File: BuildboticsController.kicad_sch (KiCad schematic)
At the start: 0 parts

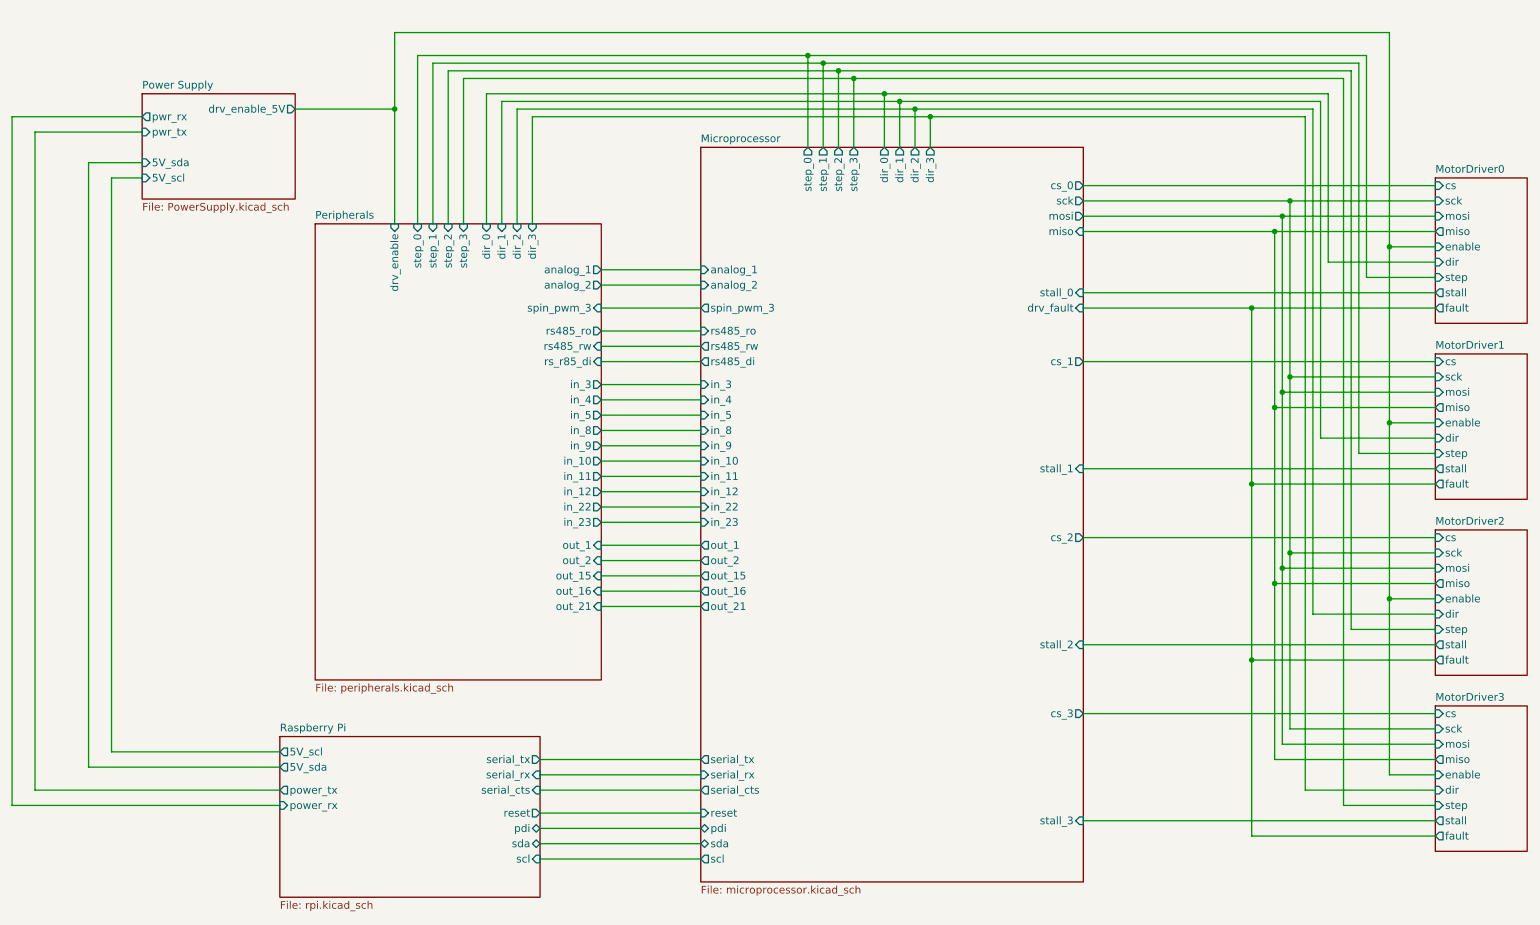
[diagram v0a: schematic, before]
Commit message: first commit of V18
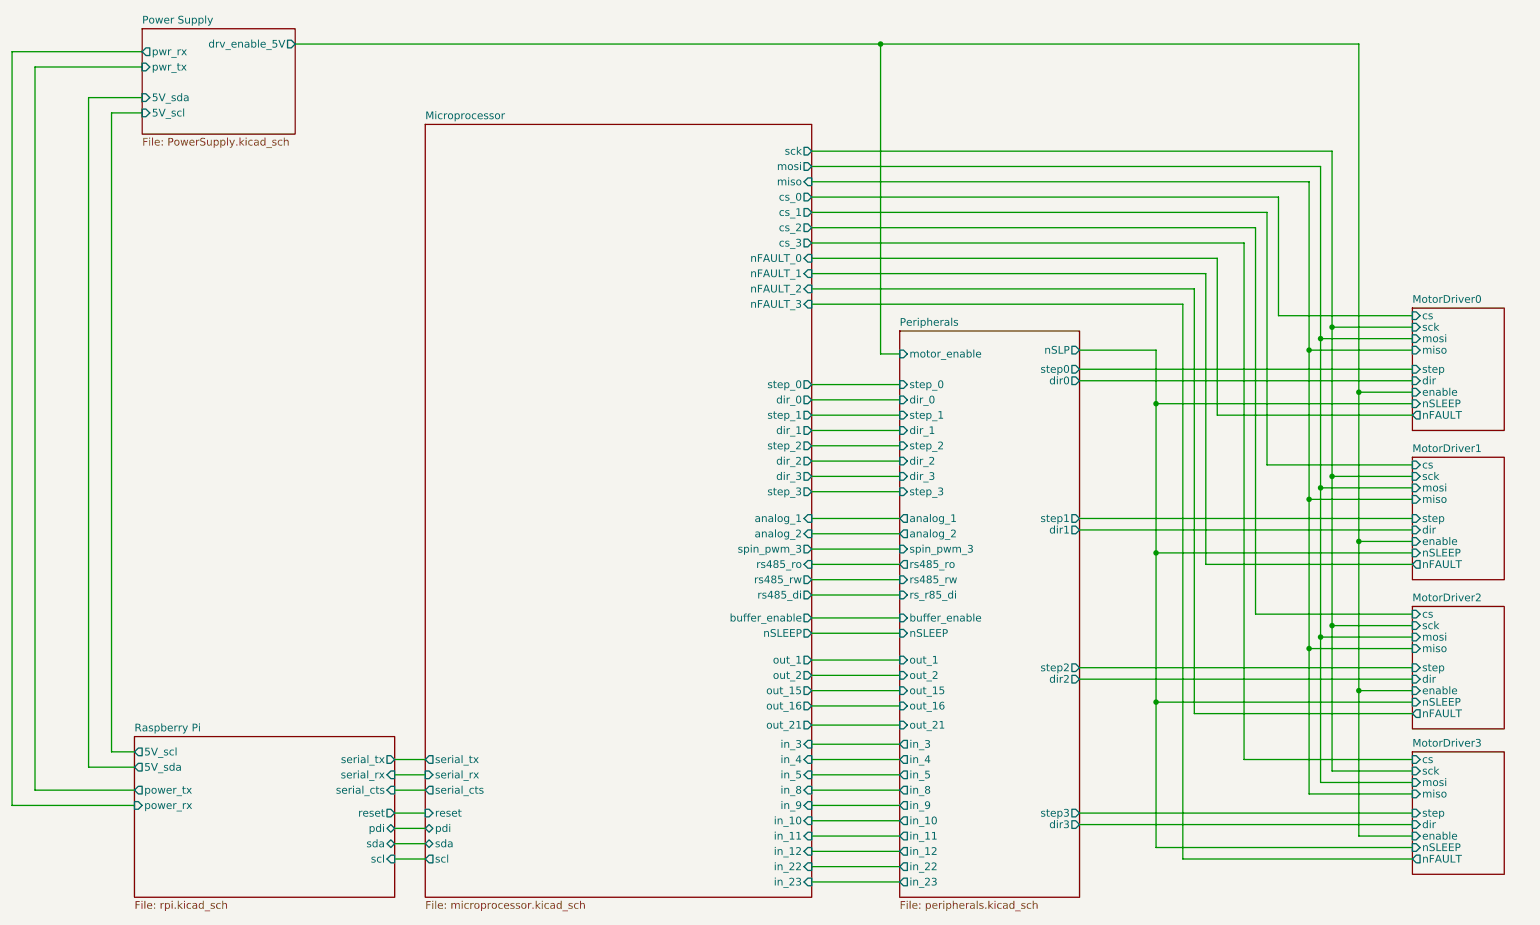
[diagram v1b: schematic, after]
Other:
- sheet Microprocessor ports: added buffer_enable, nFAULT_0, nFAULT_1, nFAULT_2, nFAULT_3, nSLEEP; removed drv_fault, stall_0, stall_1, stall_2, stall_3
- sheet MotorDriver0 ports: added nFAULT, nSLEEP; removed fault, stall
- sheet MotorDriver1 ports: added nFAULT, nSLEEP; removed fault, stall
- sheet MotorDriver2 ports: added nFAULT, nSLEEP; removed fault, stall
- sheet MotorDriver3 ports: added nFAULT, nSLEEP; removed fault, stall
- sheet Peripherals ports: added buffer_enable, dir0, dir1, dir2, dir3, motor_enable, nSLEEP, nSLP, step0, step1, step2, step3; removed drv_enable

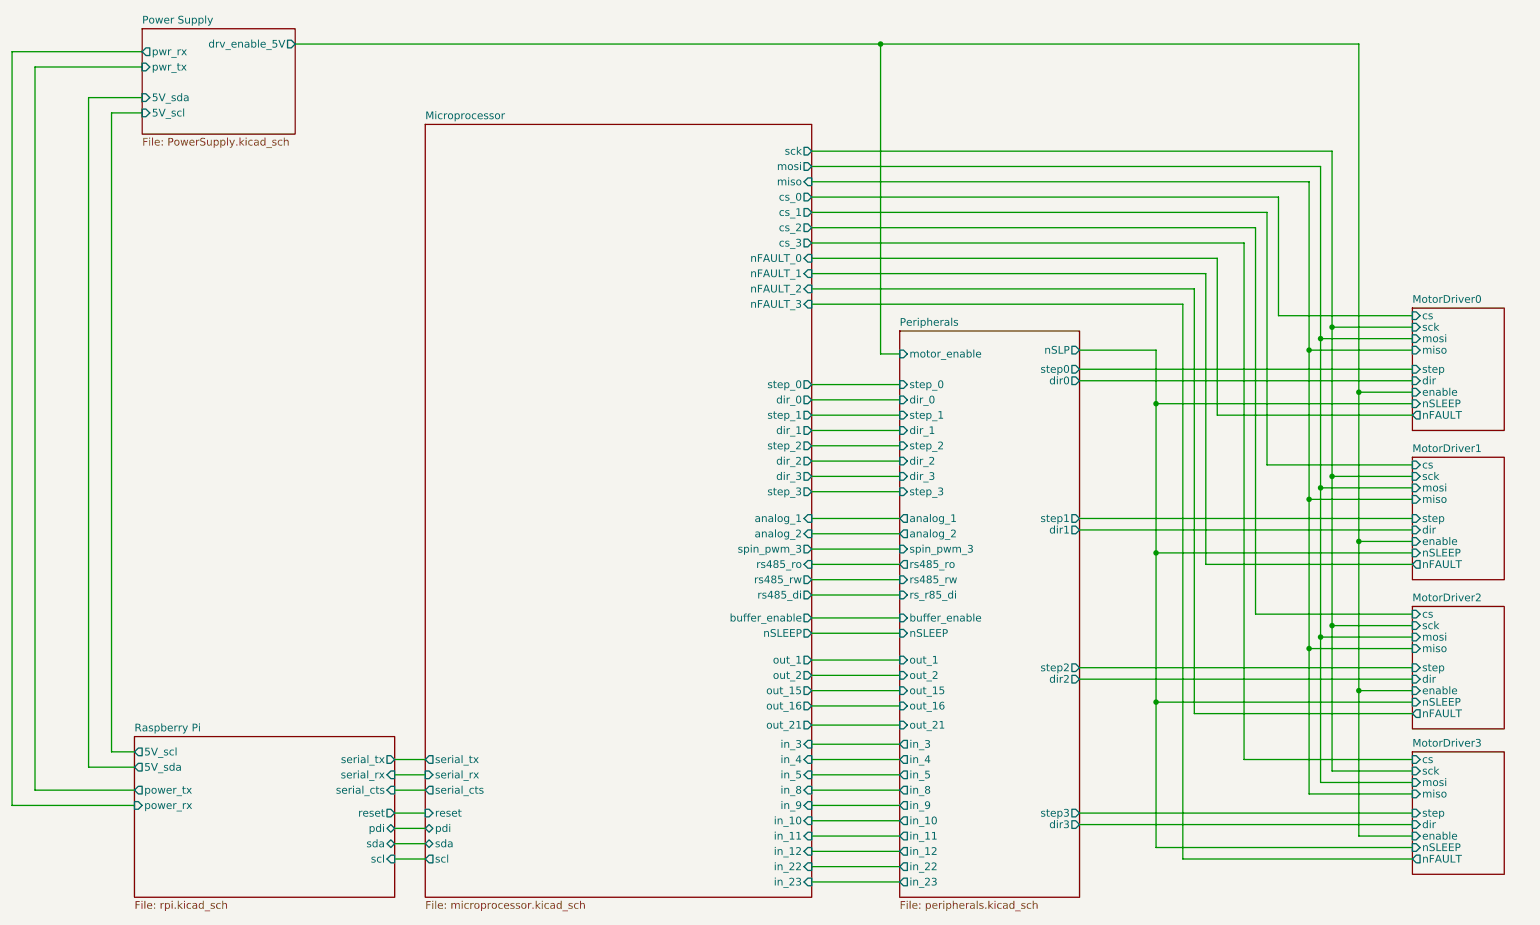
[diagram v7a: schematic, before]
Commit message: Move back to drv8711
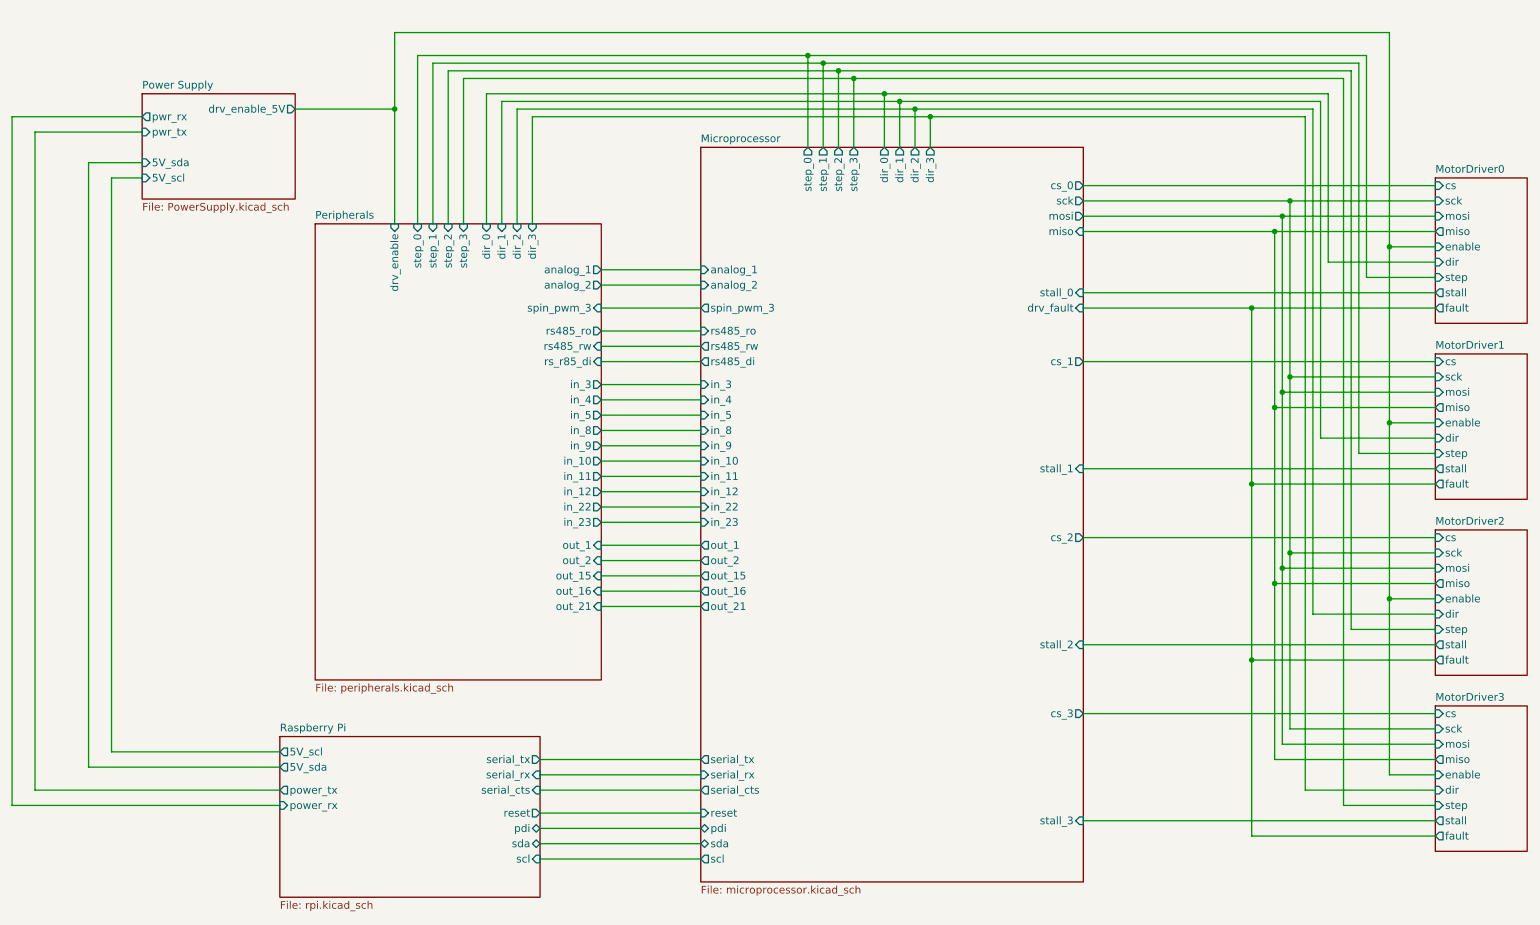
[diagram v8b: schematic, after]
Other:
- sheet Microprocessor ports: added drv_fault, stall_0, stall_1, stall_2, stall_3; removed buffer_enable, nFAULT_0, nFAULT_1, nFAULT_2, nFAULT_3, nSLEEP
- sheet MotorDriver0 ports: added fault, stall; removed nFAULT, nSLEEP
- sheet MotorDriver1 ports: added fault, stall; removed nFAULT, nSLEEP
- sheet MotorDriver2 ports: added fault, stall; removed nFAULT, nSLEEP
- sheet MotorDriver3 ports: added fault, stall; removed nFAULT, nSLEEP
- sheet Peripherals ports: added drv_enable; removed buffer_enable, dir0, dir1, dir2, dir3, motor_enable, nSLEEP, nSLP, step0, step1, step2, step3
